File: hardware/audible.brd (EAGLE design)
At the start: 27.7 x 23.4 mm, 27 parts, among them IC1 LTC1966CMS8, J1 SQUALL_HEADER, J2 HIROSE-DF40C-10DP-0.4V, J3 HIROSE-DF40C-10DP-0.4V, J5 TC2030-JLINK-NL, U1 MAX417ESA+, U2 MAX417ESA+

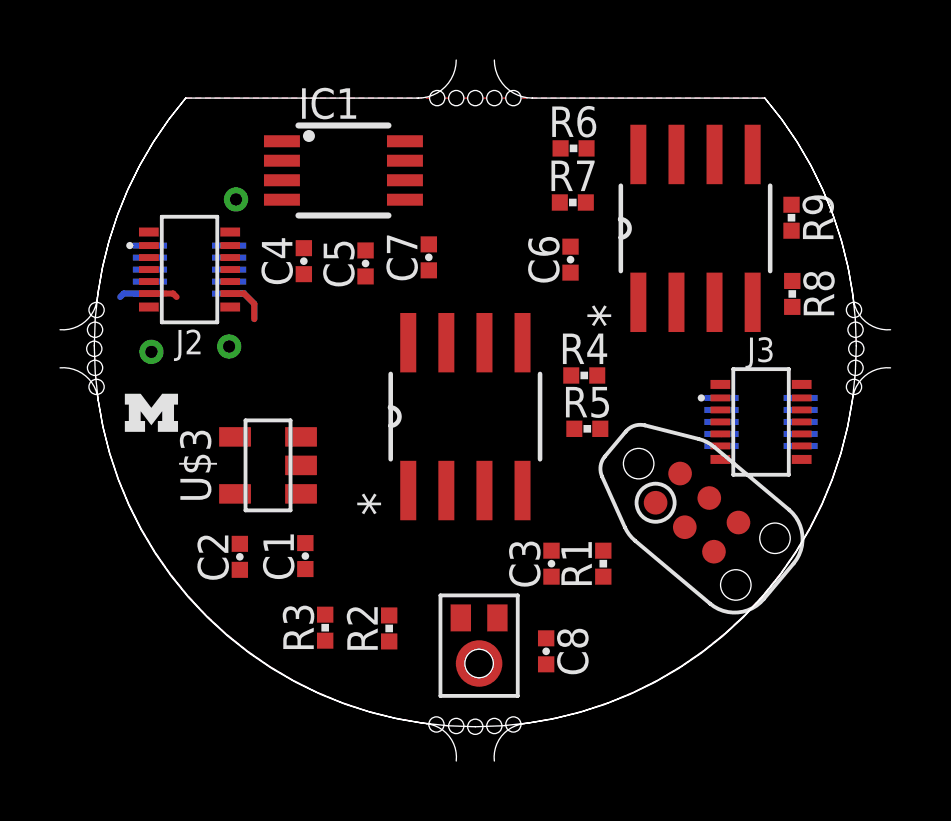
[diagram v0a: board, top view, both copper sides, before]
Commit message: better schematic
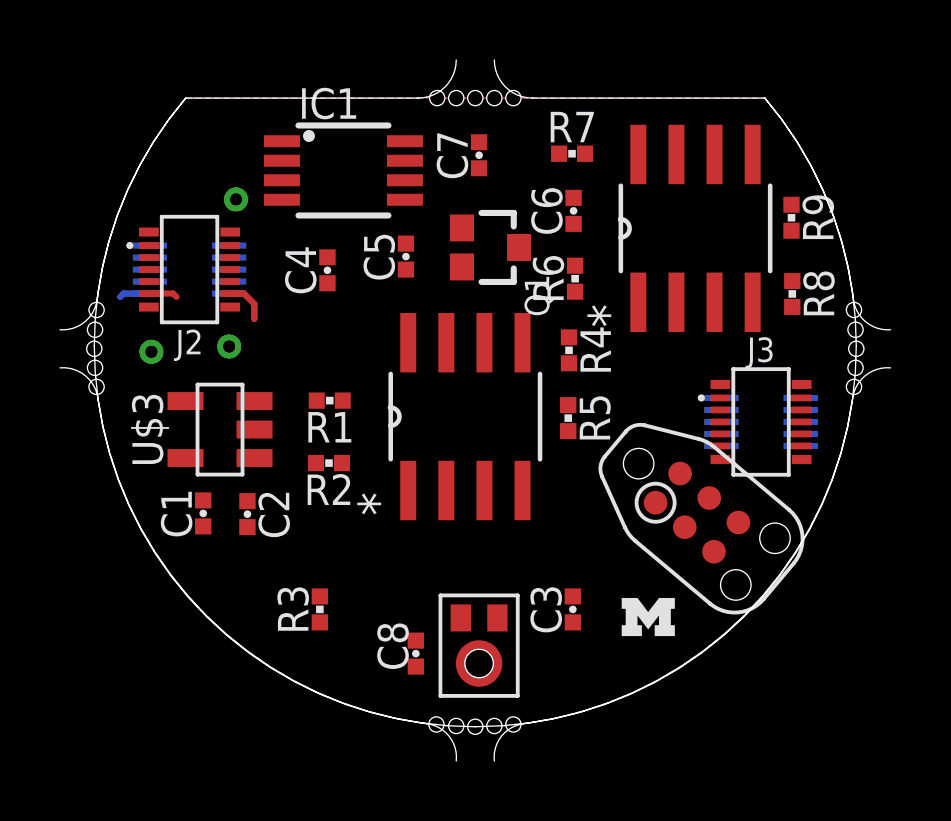
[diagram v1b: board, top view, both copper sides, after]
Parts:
- added Q1: FK3503010L, chips:SC85
- moved U$1 17.9 mm to (29.9, 3.66)
- moved R1 10.6 mm to (19.3, 10.9), turned to 180 degrees
- moved R2 5.87 mm to (19.3, 8.79), turned to 180 degrees
- moved C8 4.34 mm to (22.1, 2.44)
- moved R6 4.34 mm to (27.5, 14.9), turned to 90 degrees
- moved C7 3.79 mm to (24.3, 19.1)
- moved C1 3.69 mm to (15.1, 7.11)
- moved U$3 2.00 mm to (15.6, 9.91)
- moved C3 1.68 mm to (27.4, 3.91)
- moved C6 1.63 mm to (27.4, 17.2)
- moved R7 1.63 mm to (27.4, 19.1)
- moved C2 1.44 mm to (16.5, 7.09), turned to 270 degrees
- moved C5 1.37 mm to (21.8, 15.7)
- moved R4 0.98 mm to (27.3, 12.5), turned to 270 degrees
- moved C4 0.84 mm to (19.2, 15.2)
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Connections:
- net GND: now also Q1.2
- net N$10: now also Q1.3
- net P22: now also U$3.3
- net P24: now also Q1.1
